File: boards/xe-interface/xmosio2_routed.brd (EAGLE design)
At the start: 116.8 x 100 mm, 122 parts, among them IC1 IDTQS3245QSOP20, IC2 IDTQS3245QSOP20, IC3 IDTQS3245QSOP20, IC4 IDTQS3245QSOP20, IC5 IDTQS3245QSOP20, J1 SD_CARD, U1 24 MHz Osc. (F535L-24), X1 0446200002

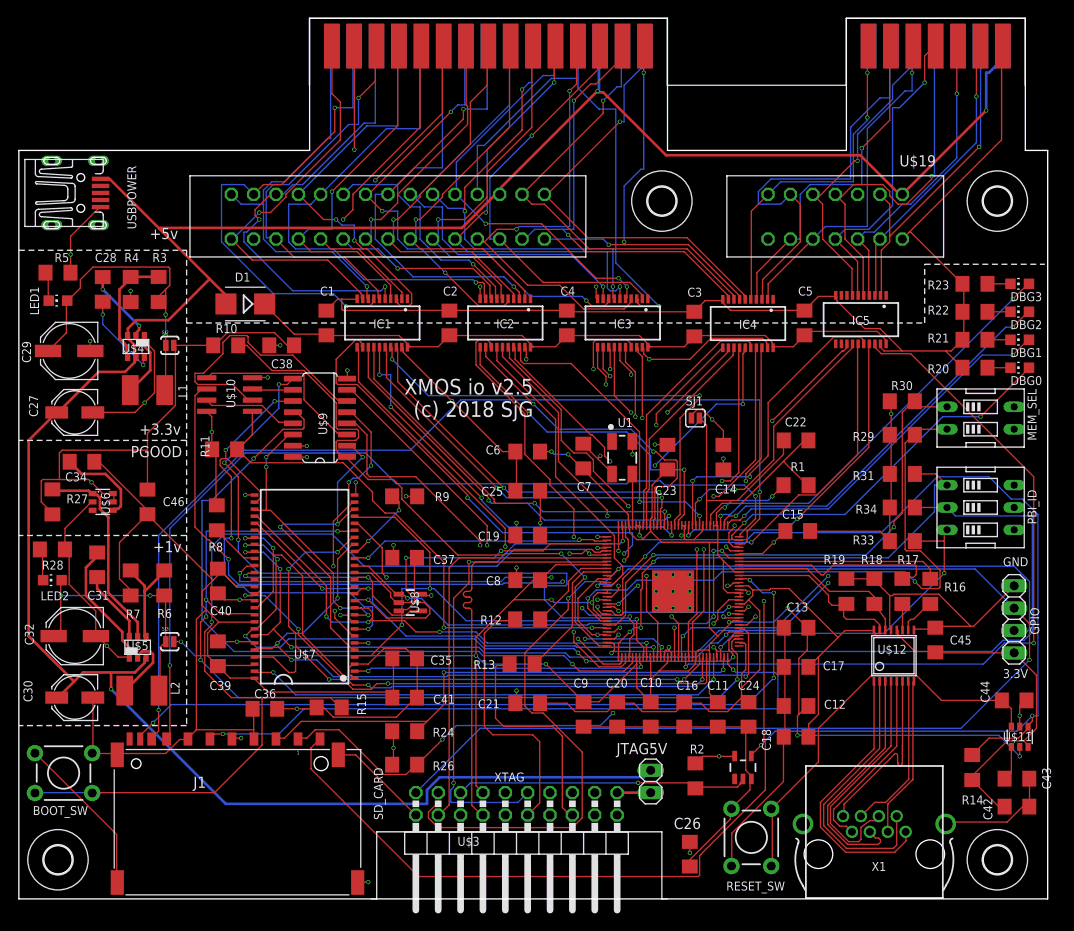
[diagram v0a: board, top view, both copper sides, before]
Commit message: Latest board files. Submitted board is xmosio2_routed.brd
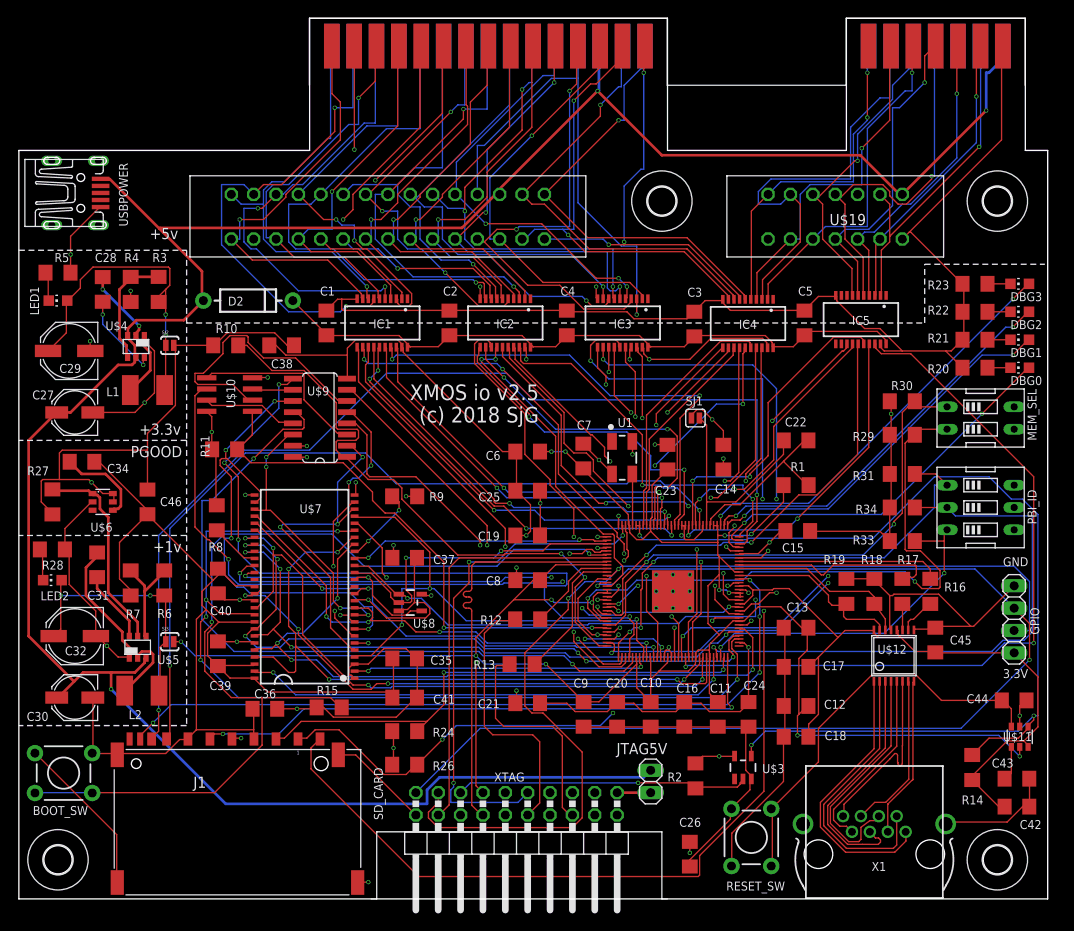
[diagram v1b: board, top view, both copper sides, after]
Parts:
- removed D1: MURS120-E3, diode:SMB
- added D2: (no value), SparkFun-DiscreteSemi:DIODE-1N4001-KIT
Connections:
- net +4.3V: now also D2.C; no longer D1.C
- net +5V: now also D2.A; no longer D1.A
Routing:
- net GND: track 586.4 -> 610.0 mm, vias 37 -> 34
- net X_D6: track 36.2 -> 52.5 mm, vias 2 -> 3
- net X_D3: track 37.9 -> 50.7 mm, vias 2 -> 3
- net VCCIO: track 295.8 -> 283.6 mm, vias 23 -> 24
- net SDC_CLK: track 76.7 -> 66.6 mm
- net !X_S4!: track 64.3 -> 57.7 mm, vias 3 -> 4
- net !SD_CAS!: track 54.8 -> 60.6 mm, vias 4 -> 3
- net SDC_CD: track 89.3 -> 85.9 mm
- net +5V: track 289.6 -> 286.4 mm
- net +4.3V: track 78.9 -> 75.9 mm
- net X_A8: track 34.1 -> 37.1 mm, vias 0 -> 2
- net !X_S5!: track 40.9 -> 38.0 mm
- net VCCINT: track 246.4 -> 243.6 mm
- net TDI: track 33.5 -> 35.6 mm
- net SDC_D1: track 115.8 -> 117.8 mm
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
